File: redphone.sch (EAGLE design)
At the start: 227 parts, among them IC1 EP4CE22U14I7N, IC10 MPU9250, IC11 PCA9633TK, IC12 BME280, IC13 W25Q64FV, IC14 MC-1010-G, IC15 MAX2659, IC2 STM32F429NI, IC20 MP34DT01, IC25 APDS-9960, IC3 MT48LC16M16A2B4, IC4 MT48LC16M16A2B4, IC5 W25Q64FV, IC6 SIM800H, IC7 TPS65217, IC8 ESP8266, IC9 WM8903, M1 VIBRO, Q1 IRLML2502, Q2 IRLML2502, Q3 IRLML2502, SW1 PWR, SW3 VOL+, SW4 VOL-, X1 USB, X2 OV5647, X3 RM68120_LCD, X4 MICRO_SIM_SDS8, X5 LG_P715_TS, X7 AUDIO-JACKSMD, X8 FPC_I9500_BAT_CON, Y1 2.4Ghz, Y3 2.4Ghz, Y4 GSM_PCB

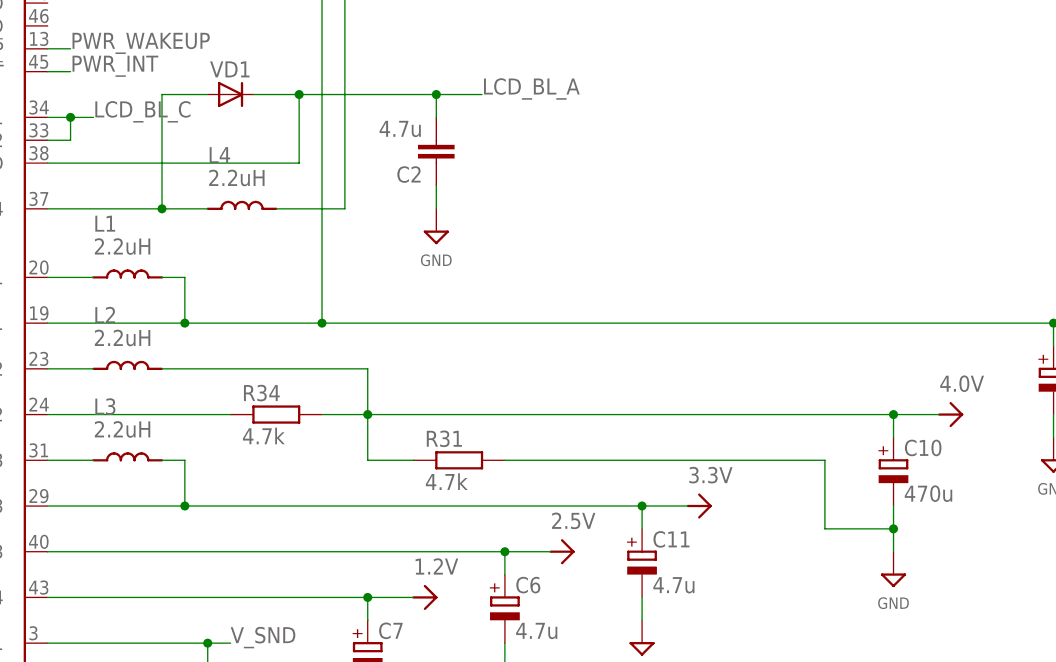
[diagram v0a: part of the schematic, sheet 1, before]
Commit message: fix DCDC2 res
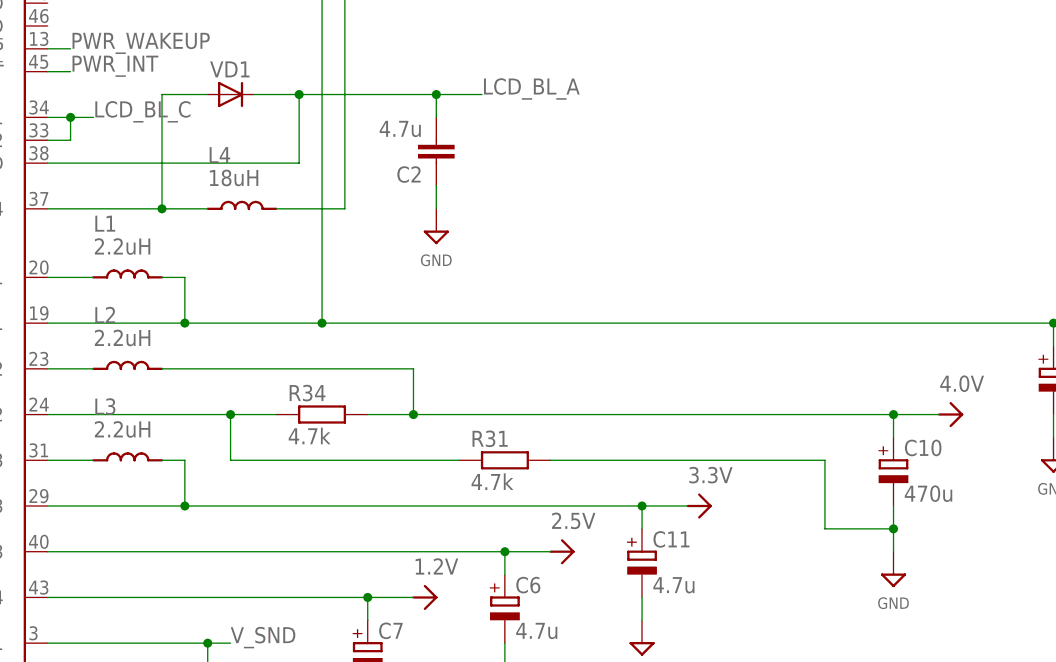
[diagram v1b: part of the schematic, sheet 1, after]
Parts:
- L4: value 2.2uH -> 18uH
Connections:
- removed net N$16: IC7.VDCDC2, R34.1
- new net N$18: IC7.VDCDC2, R31.1, R34.1
- net 4.0V: no longer R31.1
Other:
- moved on the sheet: R31, R34
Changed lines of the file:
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@@
 <part name="L2" library="netcat" deviceset="L" device="-2520" value="2.2uH"/>
 <part name="L3" library="netcat" deviceset="L" device="-2520" value="2.2uH"/>
-<part name="L4" library="netcat" deviceset="L" device="-2520" value="2.2uH"/>
+<part name="L4" library="netcat" deviceset="L" device="-2520" value="18uH"/>
 <part name="C3" library="netcat" deviceset="CAP" device="0603" value="0.1u, 6.3v"/>
 <part name="C4" library="netcat" deviceset="CAP" device="1206" value="10u, 10v"/>
@@
 <attribute name="VALUE" x="127" y="-71.12" size="1.27" layer="96" align="top-center"/>
 </instance>
-<instance part="R31" gate="G$1" x="114.3" y="-10.16" smashed="yes">
-<attribute name="NAME" x="110.49" y="-8.6614" size="1.778" layer="95"/>
-<attribute name="VALUE" x="110.49" y="-13.462" size="1.778" layer="96"/>
-</instance>
-<instance part="R34" gate="G$1" x="93.98" y="-5.08" smashed="yes">
-<attribute name="NAME" x="90.17" y="-3.5814" size="1.778" layer="95"/>
-<attribute name="VALUE" x="90.17" y="-8.382" size="1.778" layer="96"/>
+<instance part="R31" gate="G$1" x="119.38" y="-10.16" smashed="yes">
+<attribute name="NAME" x="115.57" y="-8.6614" size="1.778" layer="95"/>
+<attribute name="VALUE" x="115.57" y="-13.462" size="1.778" layer="96"/>
+</instance>
+<instance part="R34" gate="G$1" x="99.06" y="-5.08" smashed="yes">
+<attribute name="NAME" x="95.25" y="-3.5814" size="1.778" layer="95"/>
+<attribute name="VALUE" x="95.25" y="-8.382" size="1.778" layer="96"/>
 </instance>
 <instance part="R35" gate="G$1" x="0" y="30.48" smashed="yes" rot="R90">
@@
 <pinref part="R31" gate="G$1" pin="2"/>
 <wire x1="162.56" y1="-17.78" x2="162.56" y2="-20.32" width="0.1524" layer="91"/>
-<wire x1="119.38" y1="-10.16" x2="154.94" y2="-10.16" width="0.1524" layer="91"/>
+<wire x1="124.46" y1="-10.16" x2="154.94" y2="-10.16" width="0.1524" layer="91"/>
 <wire x1="154.94" y1="-10.16" x2="154.94" y2="-17.78" width="0.1524" layer="91"/>
 <wire x1="154.94" y1="-17.78" x2="162.56" y2="-17.78" width="0.1524" layer="91"/>
@@
 <pinref part="U$2" gate="G$1" pin="4.0V"/>
 <pinref part="L2" gate="G$1" pin="P$2"/>
-<wire x1="104.14" y1="-5.08" x2="162.56" y2="-5.08" width="0.1524" layer="91"/>
+<wire x1="109.22" y1="-5.08" x2="162.56" y2="-5.08" width="0.1524" layer="91"/>
 <wire x1="162.56" y1="-5.08" x2="167.64" y2="-5.08" width="0.1524" layer="91"/>
-<wire x1="81.28" y1="0" x2="104.14" y2="0" width="0.1524" layer="91"/>
-<wire x1="104.14" y1="0" x2="104.14" y2="-5.08" width="0.1524" layer="91"/>
+<wire x1="81.28" y1="0" x2="109.22" y2="0" width="0.1524" layer="91"/>
+<wire x1="109.22" y1="0" x2="109.22" y2="-5.08" width="0.1524" layer="91"/>
 <pinref part="C10" gate="G$1" pin="+"/>
 <wire x1="162.56" y1="-7.62" x2="162.56" y2="-5.08" width="0.1524" layer="91"/>
 <junction x="162.56" y="-5.08"/>
 <pinref part="R34" gate="G$1" pin="2"/>
-<wire x1="99.06" y1="-5.08" x2="104.14" y2="-5.08" width="0.1524" layer="91"/>
-<junction x="104.14" y="-5.08"/>
-<pinref part="R31" gate="G$1" pin="1"/>
-<wire x1="109.22" y1="-10.16" x2="104.14" y2="-10.16" width="0.1524" layer="91"/>
-<wire x1="104.14" y1="-10.16" x2="104.14" y2="-5.08" width="0.1524" layer="91"/>
+<wire x1="104.14" y1="-5.08" x2="109.22" y2="-5.08" width="0.1524" layer="91"/>
+<junction x="109.22" y="-5.08"/>
 </segment>
 </net>
@@
 </segment>
 </net>
-<net name="N$16" class="0">
-<segment>
+<net name="N$18" class="0">
+<segment>
+<pinref part="R31" gate="G$1" pin="1"/>
+<wire x1="114.3" y1="-10.16" x2="88.9" y2="-10.16" width="0.1524" layer="91"/>
 <pinref part="IC7" gate="G$1" pin="VDCDC2"/>
 <pinref part="R34" gate="G$1" pin="1"/>
 <wire x1="68.58" y1="-5.08" x2="88.9" y2="-5.08" width="0.1524" layer="91"/>
-</segment>
-</net>
+<wire x1="88.9" y1="-5.08" x2="93.98" y2="-5.08" width="0.1524" layer="91"/>
+<wire x1="88.9" y1="-10.16" x2="88.9" y2="-5.08" width="0.1524" layer="91"/>
+<junction x="88.9" y="-5.08"/>
+</segment>
+</net>
